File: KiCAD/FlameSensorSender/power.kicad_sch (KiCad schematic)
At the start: 26 parts, among them J5 Conn_01x06_Socket, J6 Conn_01x06_Pin, J7 6 Pin USB-C Type USB Connecto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, Q3 AO3400A, U3 TPS63802DLAR, U4 TPS63802DLAR

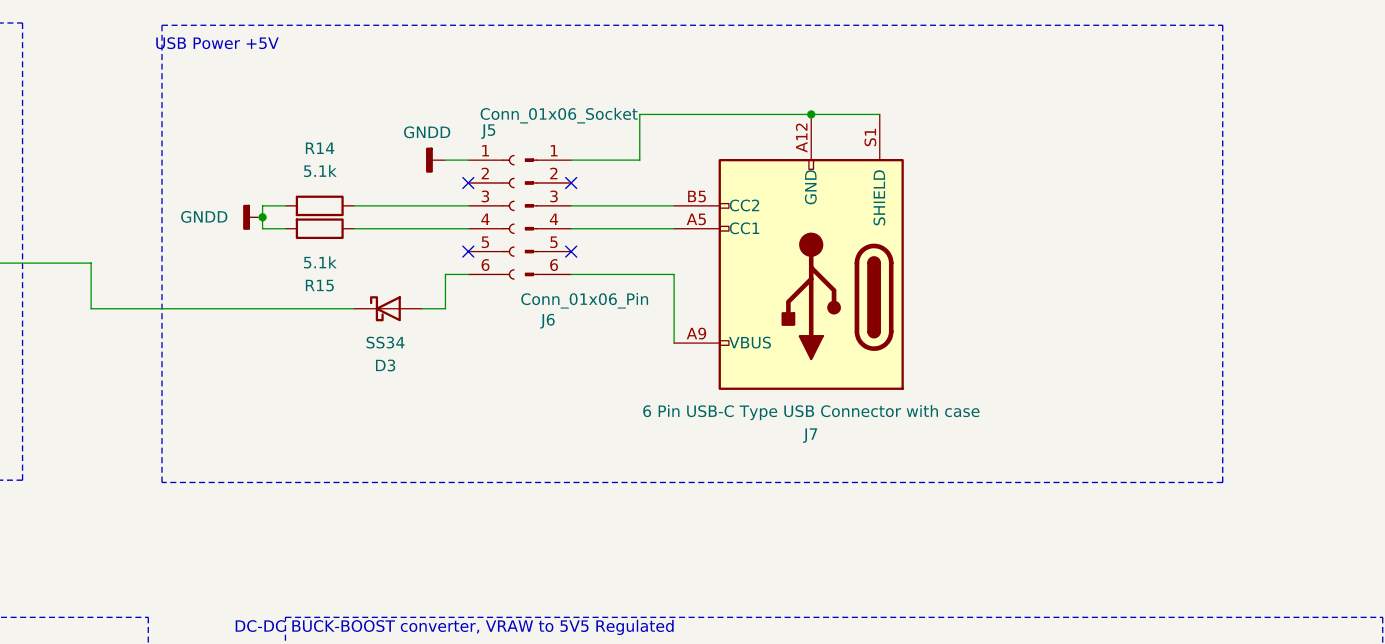
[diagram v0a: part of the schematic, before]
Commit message: lora setup done 70%
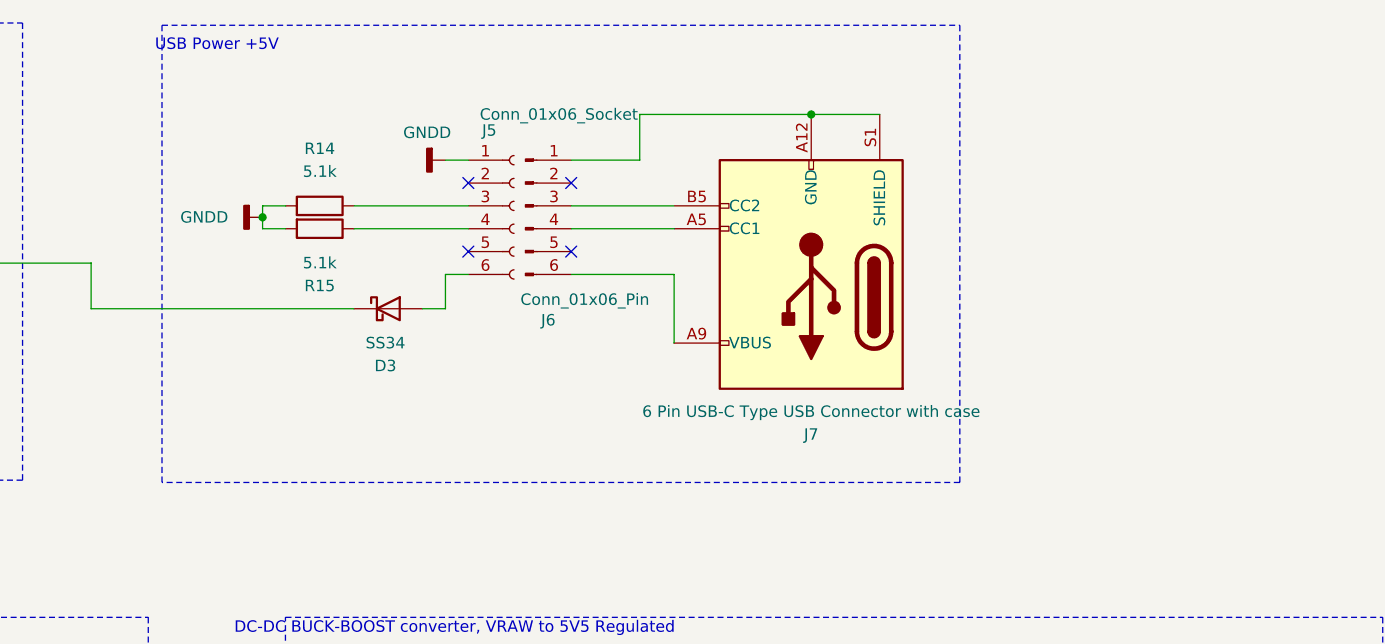
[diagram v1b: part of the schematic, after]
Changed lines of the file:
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@@
 	(rectangle
 		(start 119.634 25.654)
-		(end 237.49 76.454)
+		(end 208.28 76.454)
 		(stroke
 			(width 0)
